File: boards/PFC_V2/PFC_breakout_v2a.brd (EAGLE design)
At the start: 76.2 x 58.4 mm, 35 parts, among them CN1 1X4-BIG

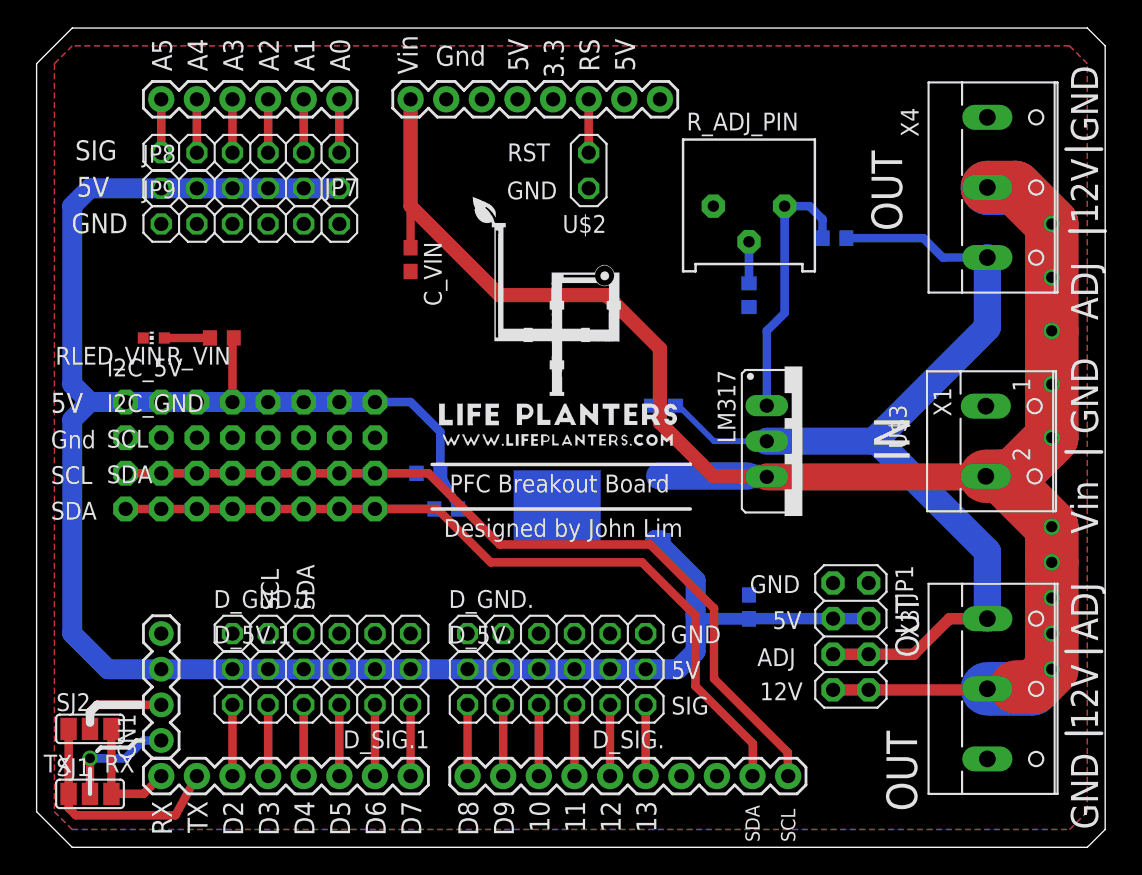
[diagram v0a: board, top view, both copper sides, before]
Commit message: boards and src
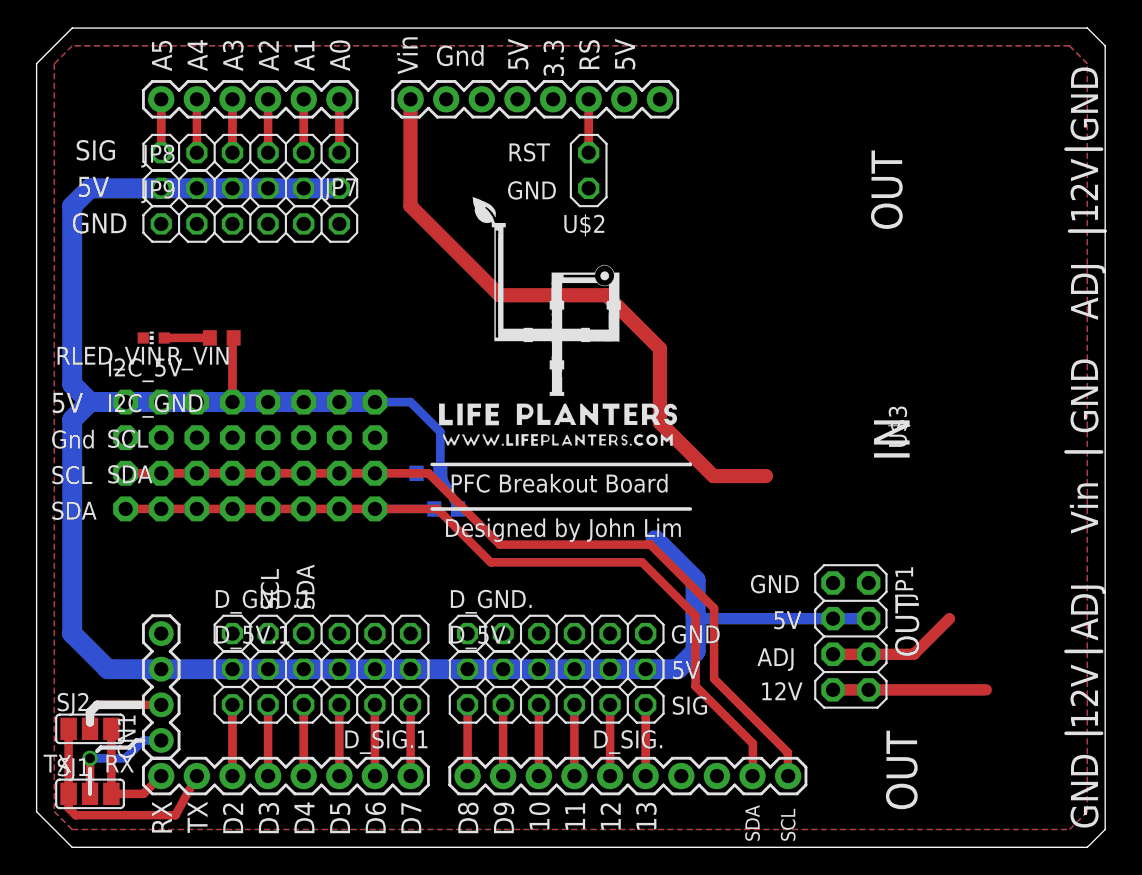
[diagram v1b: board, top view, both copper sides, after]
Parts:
- removed 5VREG: 7805DT, adafruit:TO252
- removed C_5V: 0.1uF, dp_devices:C603
- removed C_ADJ_PIN, C_VIN: 1uF, dp_devices:C603
- removed LM317: (no value), v-reg:317TS
- removed R1_VREG_PIN: 1.86k, resistor:R0603
- removed R2_VREG_PIN: 3k, resistor:R0603
- removed R_ADJ_PIN: 10K, bourns:3386P
- removed X1: (no value), con-wago-500:W237-102
- removed X3, X4: (no value), con-wago-500:W237-103
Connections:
- removed net N$23: LM317.1, R1_VREG_PIN.1, R_ADJ_PIN.3
- removed net N$24: R2_VREG_PIN.2, R_ADJ_PIN.2
- net 5V: no longer 5VREG.2, C_5V.1
- net GND: no longer 5VREG.3, C_5V.2, C_ADJ_PIN.2, C_VIN.2, R2_VREG_PIN.1, X1.1, X3.3, X4.1
- net VIN: no longer 5VREG.1, C_VIN.1, LM317.3, X1.2, X3.2, X4.2
- net V_ADJ: no longer C_ADJ_PIN.1, LM317.2, R1_VREG_PIN.2, X3.1, X4.3
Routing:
- net VIN: track 172.2 -> 55.0 mm, vias 10 -> 0
- net V_ADJ: track 70.5 -> 9.35 mm
- net N$23: track 19.2 -> 0.00 mm
- net 5V: track 159.2 -> 155.3 mm
- net N$24: track 2.96 -> 0.00 mm
